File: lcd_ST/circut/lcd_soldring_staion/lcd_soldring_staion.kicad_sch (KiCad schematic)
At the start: 36 parts, among them J1 DIN-5, J2 Conn_01x05_Pin, J3 Conn_01x01_Pin, J4 Conn_01x01_Pin, J44 Screw_Terminal_01x02, J5 Conn_01x01_Pin, J6 Conn_01x01_Pin, J7 Conn_01x04_Pin, Q2 Si4162DY, SW1 SW_Push, U1 PIC16F15223T-I/SL, U2 L7805, U3 LM358

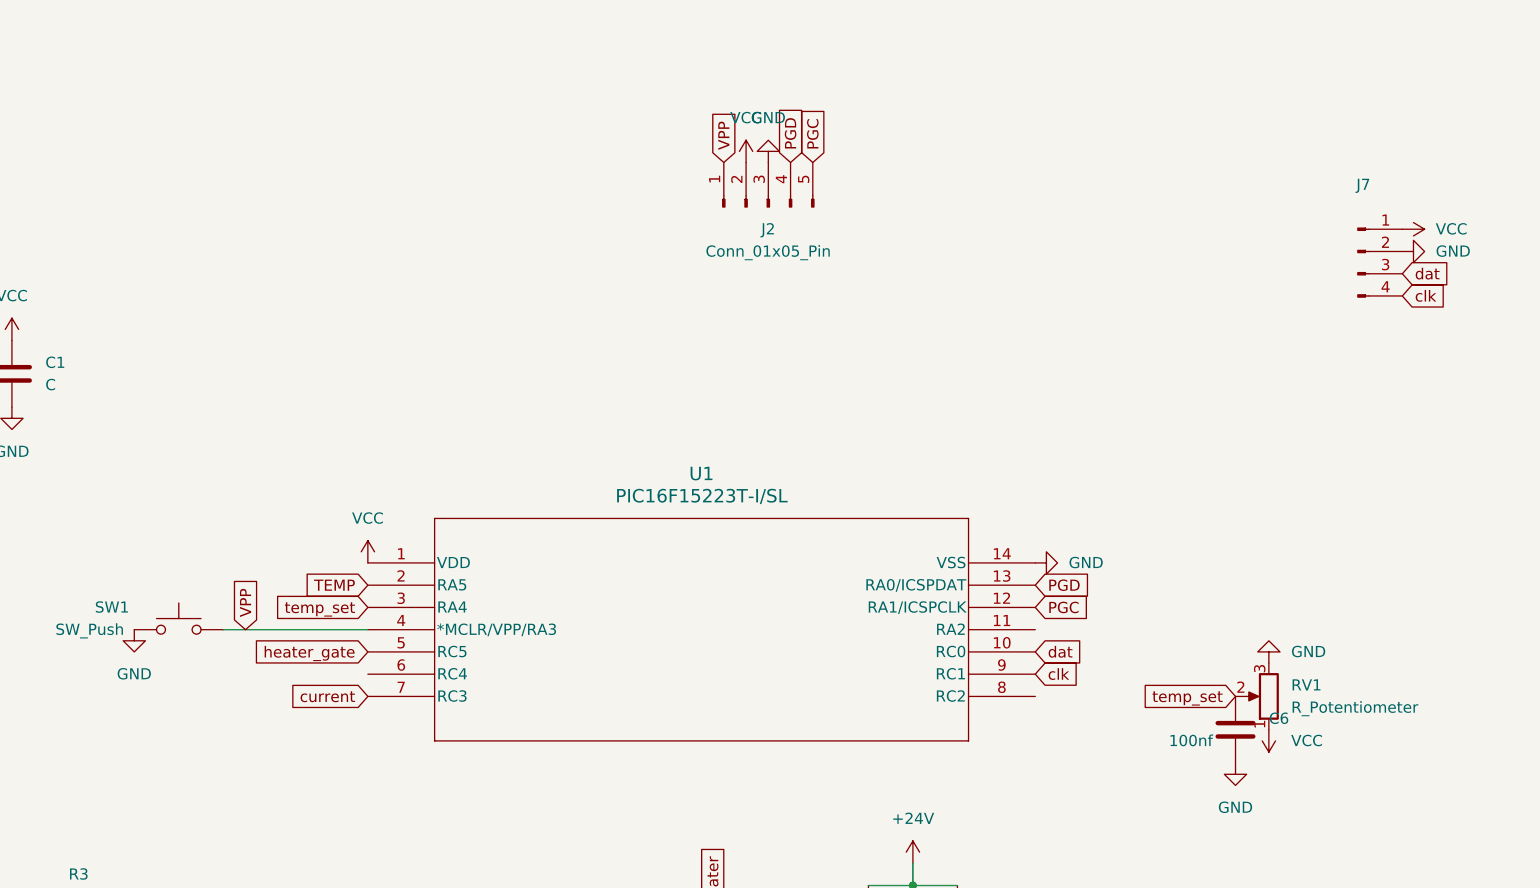
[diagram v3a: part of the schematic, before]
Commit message: V2_PCB EDITING
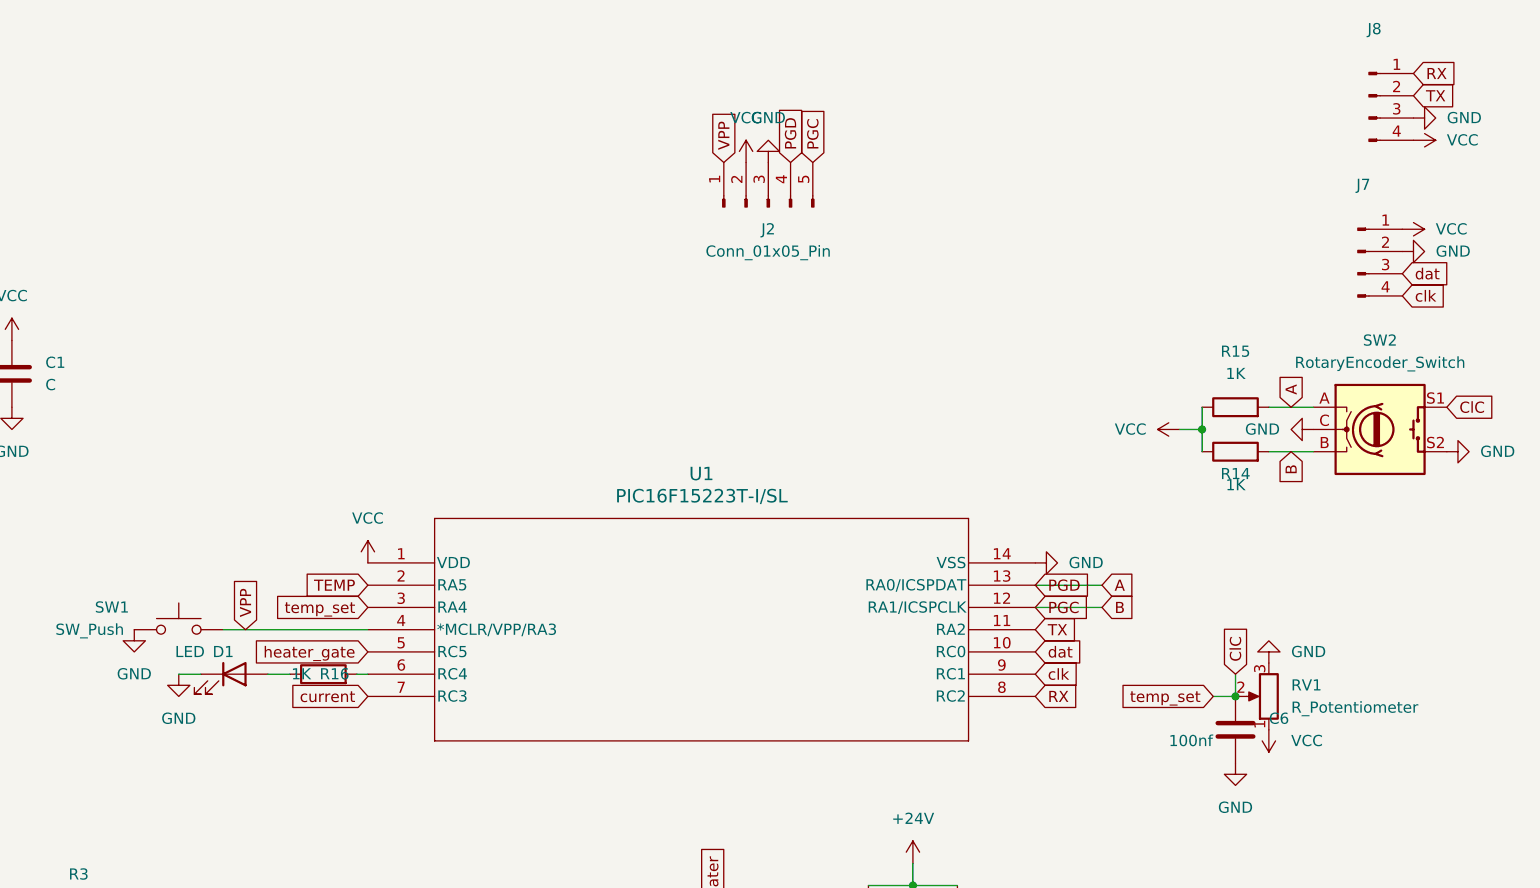
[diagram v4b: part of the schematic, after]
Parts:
- added D1: LED, LED_SMD:LED_0805_2012Metric_Pad1.15x1.40mm_HandSolder, symbol Device:LED
- added J8: Conn_01x04_Pin, Connector:FanPinHeader_1x04_P2.54mm_Vertical, symbol Connector:Conn_01x04_Pin
- added R14, R15, R16: 1K, Resistor_SMD:R_1206_3216Metric_Pad1.30x1.75mm_HandSolder, symbol Device:R
- added SW2: RotaryEncoder_Switch, symbol Device:RotaryEncoder_Switch
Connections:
- net GND: now also D1.1 (K), J8.3 (Pin_3), SW2.C, SW2.S2
- net VCC: now also J8.4 (Pin_4), R14.1, R15.1
- net TX: now reaches U1.11 (RA2)
- net TX: now also J8.2 (Pin_2)
- net at U1.6 (RC4): now also R16.2
- net RX: now reaches U1.8 (RC2)
- net RX: now also J8.1 (Pin_1)
- net PGC renamed B
- net B: now also R14.2, SW2.B
- net PGD renamed A
- net A: now also R15.2, SW2.A
- net temp_set renamed ClC
- net ClC: now also SW2.S1
- new net: D1.2 (A), R16.1
